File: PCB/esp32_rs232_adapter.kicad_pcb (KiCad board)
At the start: 2 copper layers, 46.5 x 57.7 mm, 46 parts, among them J1 Conn_01x04_Male, J2 DB9, J4 USB_B_Micro, Q1 IRF7404, SW1 Flash, SW2 Null_Modem_Selector, SW3 SW_SPST, U1 ESP32-WROOM-32D, U2 MAX3232, U3 TP4056, U4 AMS1117

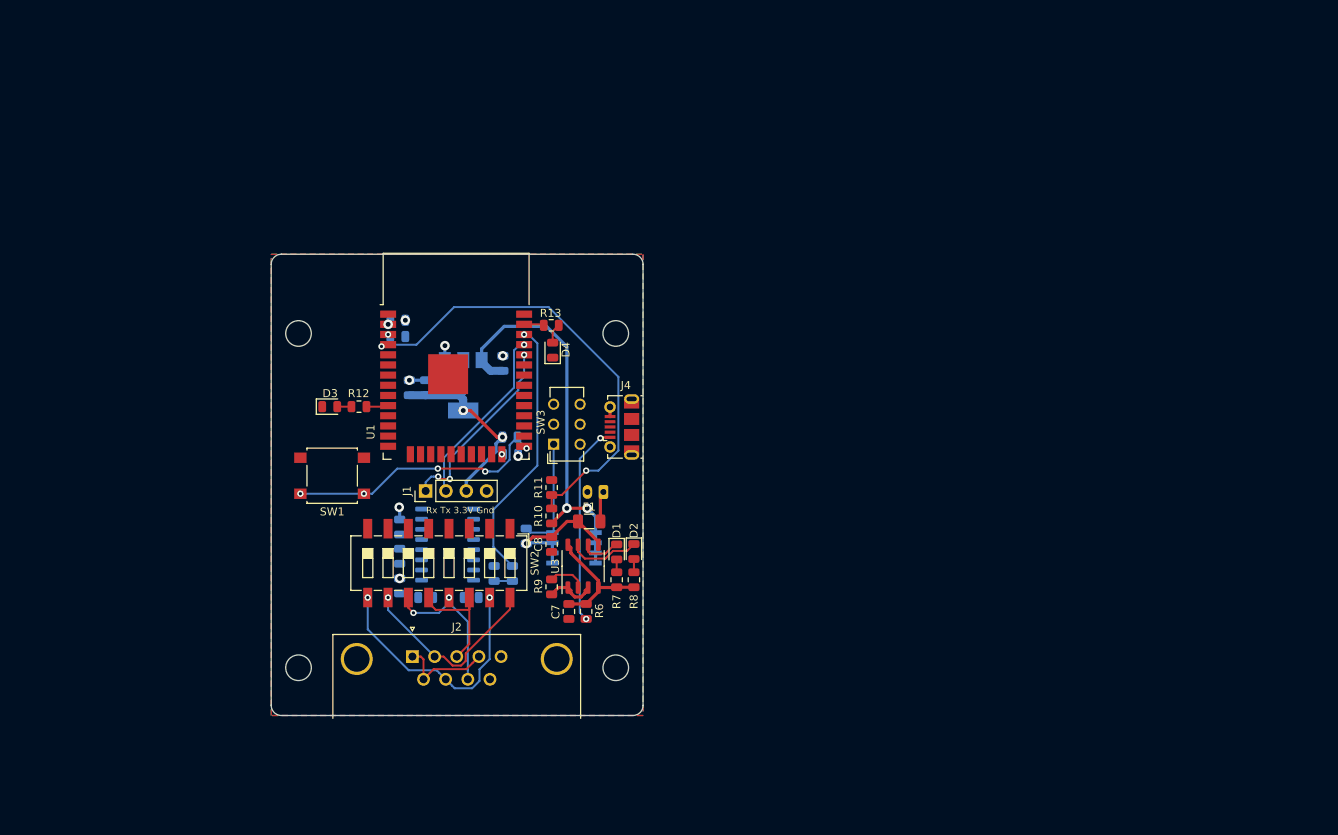
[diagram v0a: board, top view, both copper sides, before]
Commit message: work in progress with stuff for cb testing
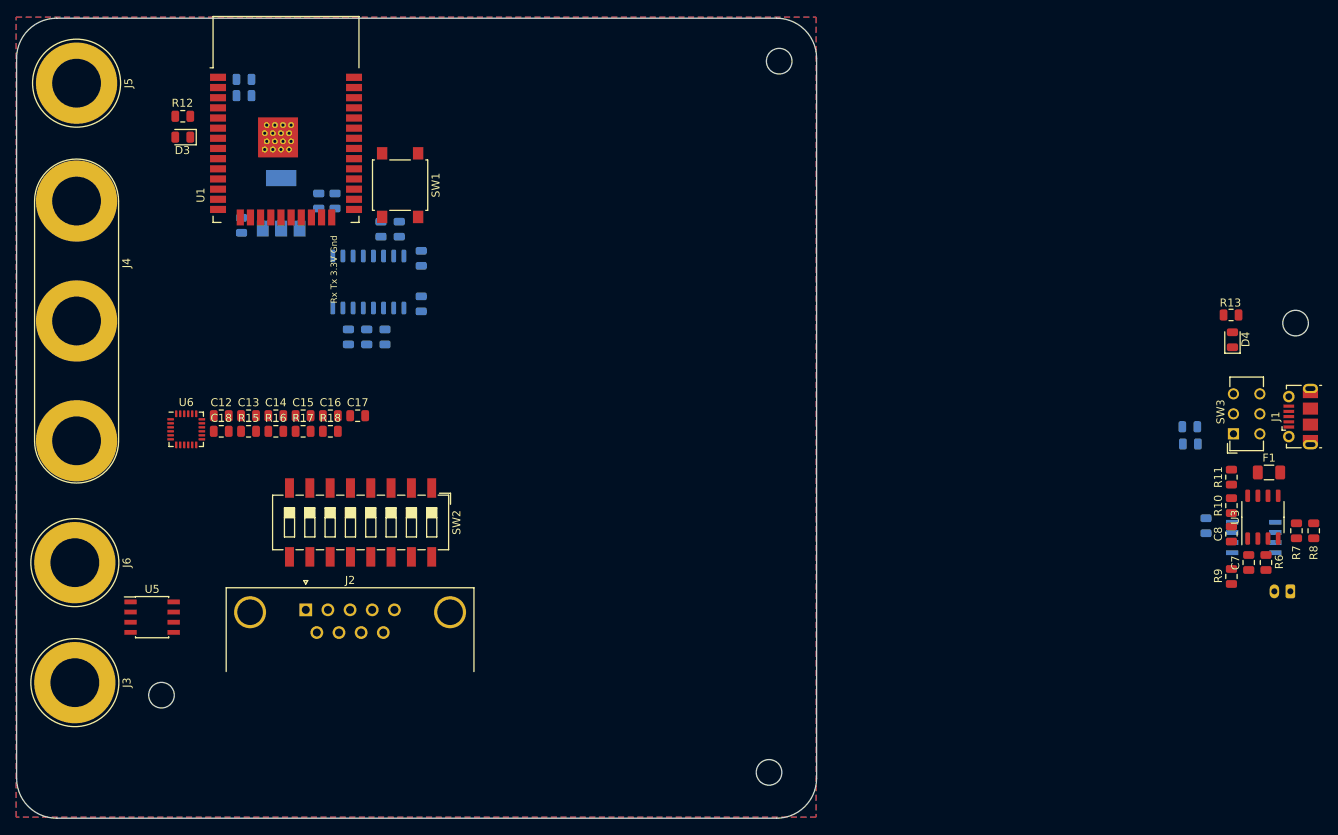
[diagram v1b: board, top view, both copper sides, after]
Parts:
- removed D1: GREEN_LED, LED_SMD:LED_0805_2012Metric
- removed D2: RED_LED, LED_SMD:LED_0805_2012Metric
- added C12: 0.1uF, Capacitor_SMD:C_0805_2012Metric, F.Cu at (125.6, 99.7)
- added C13: 1nF, Capacitor_SMD:C_0805_2012Metric, F.Cu at (129.0, 99.7)
- added C14: 0.1uF, Capacitor_SMD:C_0805_2012Metric, F.Cu at (132.4, 99.7)
- added C15: 10nF, Capacitor_SMD:C_0805_2012Metric, F.Cu at (135.8, 99.7)
- added C16: 0.1nF, Capacitor_SMD:C_0805_2012Metric, F.Cu at (139.2, 99.7)
- added C17: 0.1uF, Capacitor_SMD:C_0805_2012Metric, F.Cu at (142.6, 99.7)
- added C18: 2.2nF, Capacitor_SMD:C_0805_2012Metric, F.Cu at (125.6, 101.6)
- added J3: Shunt-, Connector:Banana_Jack_1Pin, F.Cu at (107.3, 133.1)
- added J5: Common, Connector:Banana_Jack_1Pin, F.Cu at (107.5, 58.1)
- added J6: Shunt+, Connector:Banana_Jack_1Pin, F.Cu at (107.3, 118.1)
- added R15: 3k3, Resistor_SMD:R_0805_2012Metric, F.Cu at (129.0, 101.6)
- added R16: 10k, Resistor_SMD:R_0805_2012Metric, F.Cu at (132.4, 101.6)
- added R17: 10k, Resistor_SMD:R_0805_2012Metric, F.Cu at (135.8, 101.6)
- added R18: 10k, Resistor_SMD:R_0805_2012Metric, F.Cu at (139.2, 101.6)
- added U5: ACS712xLCTR-30A, Package_SO:SOIC-8_3.9x4.9mm_P1.27mm, F.Cu at (116.9, 124.9)
- added U6: MPU-6050, Sensor_Motion:InvenSense_QFN-24_4x4mm_P0.5mm, F.Cu at (121.2, 101.4)
- C10: value 10n -> 1u
- C11: value 1u -> 10n
- J1: value Conn_01x04_Male -> USB_B_Micro; footprint Connector_PinHeader_2.54mm:PinHeader_1x04_P2.54mm_Vertical -> power_supplies:USB_Micro-B_Molex-105017-0001
- J4: value USB_B_Micro -> Poles; footprint power_supplies:USB_Micro-B_Molex-105017-0001 -> Connector:Banana_Jack_3Pin
- U1: footprint RF_Module:ESP32-WROOM-32 -> power_supplies:ESP32-WROOM-32-Heat
- moved J1 109.8 mm to (260.5, 99.8)
- moved BT1 86.8 mm to (259.2, 121.6)
- moved R6 85.2 mm to (256.2, 118.0)
- moved R7 85.2 mm to (260.0, 114.1)
- moved R8 85.2 mm to (262.1, 114.1)
- moved C7 85.2 mm to (254.0, 118.0)
- moved F1 85.2 mm to (256.6, 106.8)
- moved U3 85.2 mm to (255.8, 112.4)
- moved C8 85.0 mm to (251.9, 114.5)
- moved R10 85.0 mm to (251.9, 110.9)
- moved R11 85.0 mm to (251.9, 107.4)
- moved R9 85.0 mm to (251.9, 119.8)
- moved D4 85.0 mm to (252.0, 90.2)
- moved Q1 85.0 mm to (254.6, 114.9)
- moved R13 85.0 mm to (251.8, 87.1)
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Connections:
- J1 pad 1: /RXD -> /power_supply/P5_0
- J1 pad 2: /TXD -> (no net)
- J1 pad 3: +3V3 -> (no net)
- J1 pad 4: GND -> (no net)
- J2 pad 9: Net-(J2-Pad9) -> (no net)
- J4 pad 1: /power_supply/P5_0 -> /Aph
- J4 pad 2: Net-(J4-Pad2) -> /Bph
- J4 pad 3: Net-(J4-Pad3) -> /Cph
- R10 pad 1: /power_supply/P_Batt_1 -> +BATT
- R10 pad 2: /power_supply/Vbatt_sig -> Net-(Q1-Pad4)
- R11 pad 1: /power_supply/Vbatt_sig -> /power_supply/P_Batt_1
- R11 pad 2: GND -> /Vbatt_sig
- R14 pad 1: +BATT -> /Vbatt_sig
- R14 pad 2: Net-(Q1-Pad4) -> GND
- R7 pad 2: Net-(D1-Pad2) -> /ChargePwrStatus
- R8 pad 2: Net-(D2-Pad2) -> /ChargeStatus
- U1 pad 10: Net-(R12-Pad1) -> /Aph
- U1 pad 11: Net-(U1-Pad11) -> /Bph
- U1 pad 12: Net-(U1-Pad12) -> /Cph
- U1 pad 13: Net-(U1-Pad13) -> (no net)
- U1 pad 14: Net-(U1-Pad14) -> /I_sense
- U1 pad 16: Net-(U1-Pad16) -> (no net)
- U1 pad 17: Net-(U1-Pad17) -> (no net)
- U1 pad 18: Net-(U1-Pad18) -> (no net)
- U1 pad 19: Net-(U1-Pad19) -> (no net)
- U1 pad 20: Net-(U1-Pad20) -> (no net)
- U1 pad 21: Net-(U1-Pad21) -> (no net)
- U1 pad 22: Net-(U1-Pad22) -> (no net)
- U1 pad 23: Net-(U1-Pad23) -> (no net)
- U1 pad 26: Net-(U1-Pad26) -> (no net)
- U1 pad 27: Net-(U1-Pad27) -> (no net)
- U1 pad 28: Net-(U1-Pad28) -> /Vbatt_sig
- U1 pad 29: Net-(U1-Pad29) -> (no net)
- U1 pad 30: Net-(U1-Pad30) -> /ChargeStatus
- U1 pad 32: Net-(U1-Pad32) -> (no net)
- U1 pad 33: Net-(U1-Pad33) -> /ChargePwrStatus
- U1 pad 37: Net-(R13-Pad1) -> (no net)
- U1 pad 4: /power_supply/Vbatt_sig -> Net-(R13-Pad1)
- U1 pad 5: Net-(U1-Pad5) -> Net-(R12-Pad1)
- U1 pad 6: Net-(U1-Pad6) -> /mpu_SCL
- U1 pad 7: Net-(U1-Pad7) -> /mpu_INT
- U1 pad 8: Net-(U1-Pad8) -> /mpu_SDA
- U1 pad 9: Net-(U1-Pad9) -> (no net)
- U3 pad 6: Net-(D1-Pad1) -> /ChargePwrStatus
- U3 pad 7: /power_supply/charge_status -> /ChargeStatus
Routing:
- net /power_supply/Vbatt_sig: track 56.8 -> 0.00 mm, vias 2 -> 0
- net /power_supply/P_Batt_1: track 50.4 -> 0.00 mm, vias 2 -> 0
- net Net-(R3-Pad2): track 33.3 -> 0.00 mm, vias 5 -> 0
- net /RTS: track 33.2 -> 0.00 mm, vias 1 -> 0
- net Net-(J2-Pad7): track 32.3 -> 0.00 mm, vias 2 -> 0
- net +3V3: track 30.7 -> 0.00 mm, vias 3 -> 0
- net /power_supply/P5_0: track 25.2 -> 0.00 mm, vias 2 -> 0
- net Net-(J2-Pad2): track 24.6 -> 0.00 mm, vias 1 -> 0
- net /RXD: track 23.9 -> 0.00 mm, vias 3 -> 0
- net /TXD: track 22.9 -> 0.00 mm, vias 1 -> 0
- net Net-(J2-Pad8): track 18.3 -> 0.00 mm, vias 2 -> 0
- net +BATT: track 17.8 -> 0.00 mm, vias 1 -> 0
- net /power_supply/P5_1: track 16.2 -> 0.00 mm
- net Net-(J2-Pad3): track 15.6 -> 0.00 mm
- net Net-(Q1-Pad4): track 14.6 -> 0.00 mm
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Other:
- board size 46.5 x 57.7 mm -> 100 x 100 mm
- net class SuperPower added: clearance 0.3, trace_width 2.2, via_dia 2.5, via_drill 1
